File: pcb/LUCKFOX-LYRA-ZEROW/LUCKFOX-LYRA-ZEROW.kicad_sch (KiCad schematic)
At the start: 73 parts, among them J1 Conn_01x07, J2 Conn_01x05, J3 Conn_01x07, J4 Conn_01x05, J5 Conn_01x05, U1 Luckfox_Lyra_Zero_W, U10 RAA211403, U11 SN74LVC1G74DCUT, U12 74LVC2G66, U13 TPS3839G33DBZT, U14 74AUP2G34GW,125, U2 CORE52840, U3 MAX3051, U4 MCP2518FD-xQBB, U5 MAX3051, U6 MAX3051, U7 MCP2518FD-xQBB, U8 MAX3051, U9 74AUP2G34GW,125, Y4 Crystal_GND24_Small, Y5 Crystal_GND24_Small

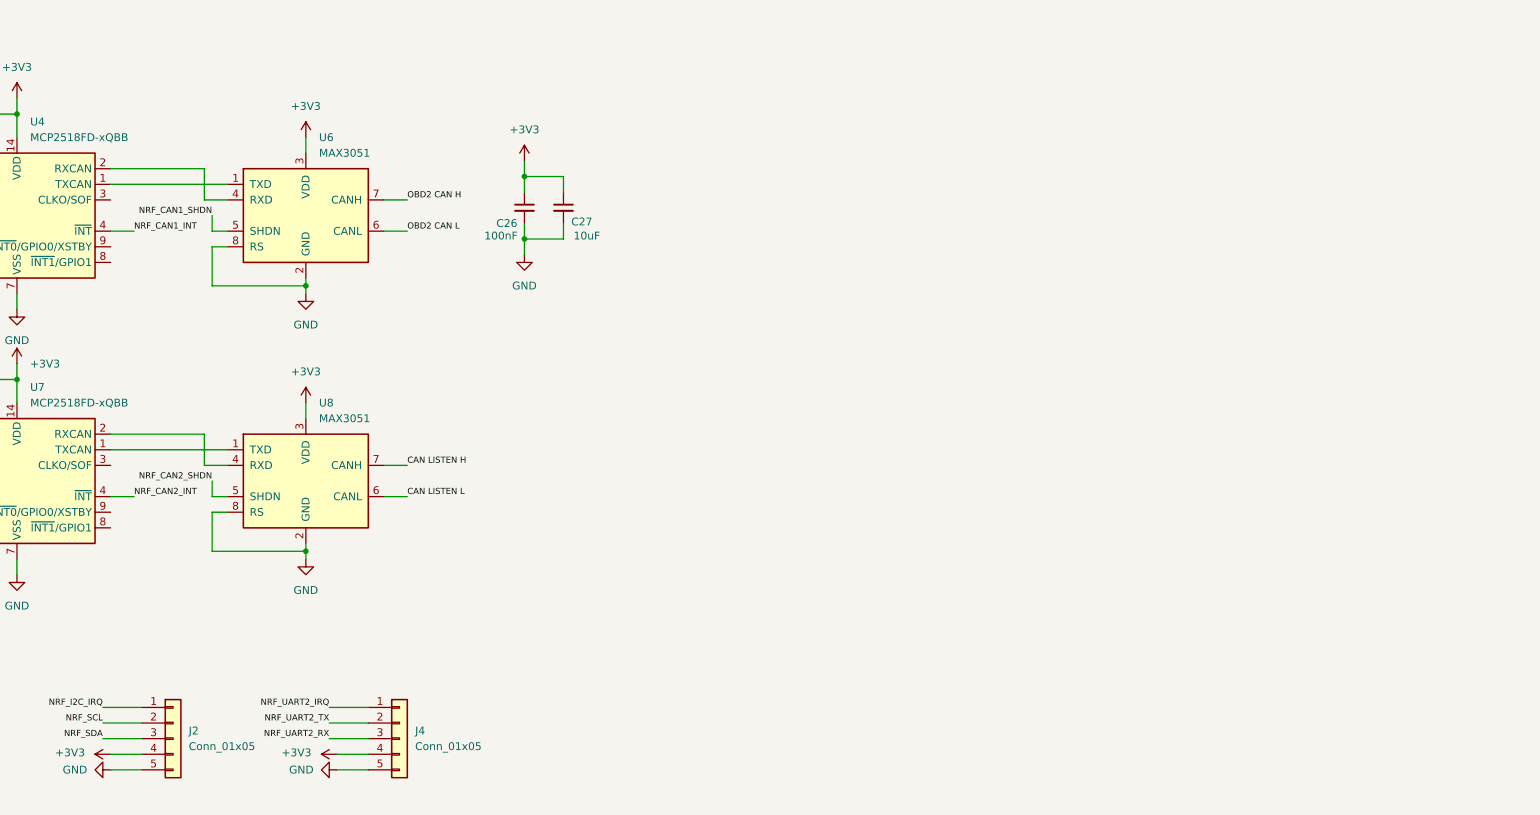
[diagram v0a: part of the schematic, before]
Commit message: fix mcp on pcb
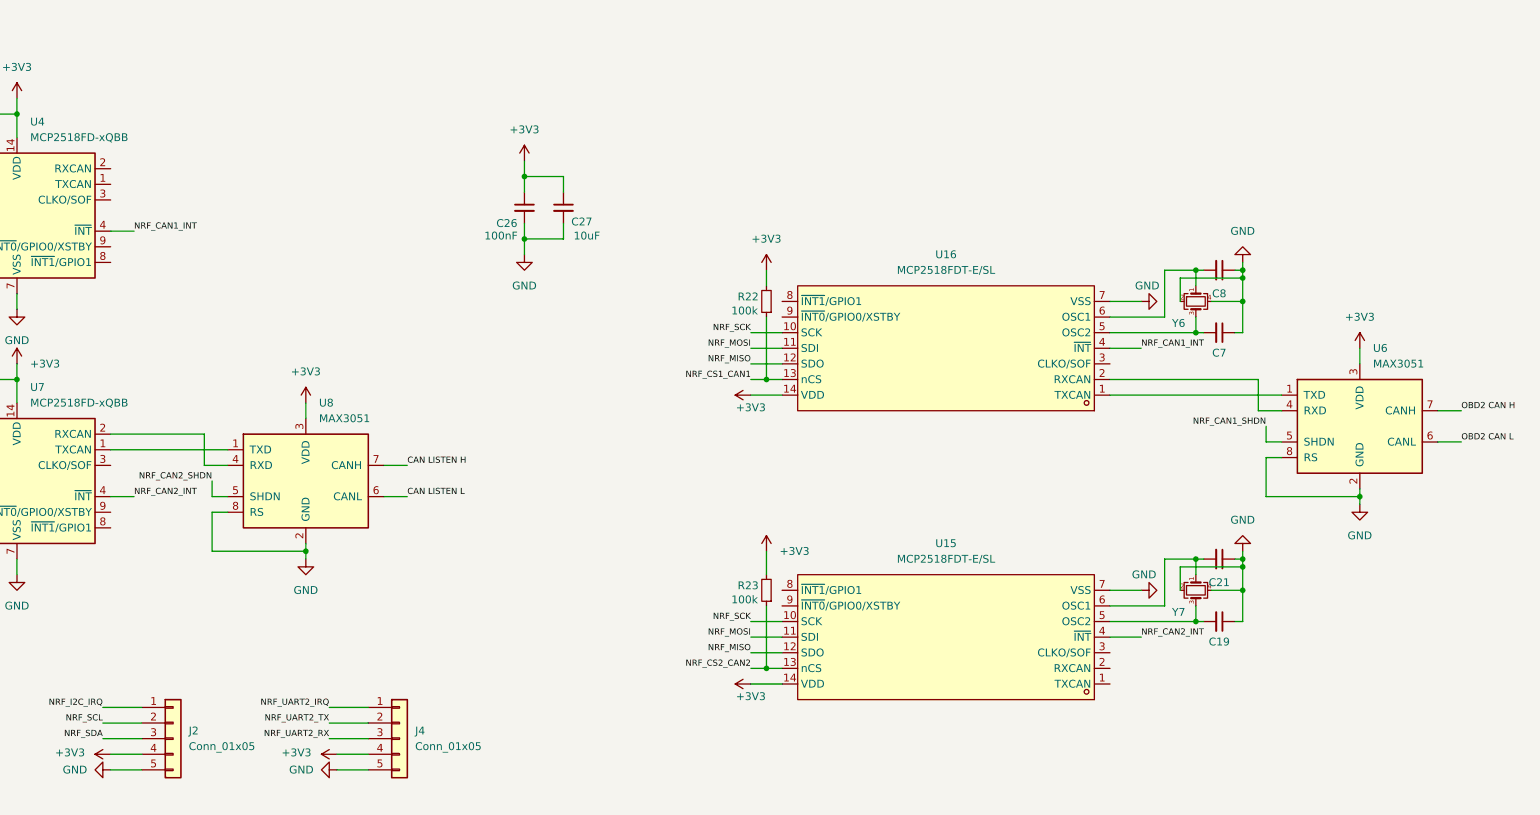
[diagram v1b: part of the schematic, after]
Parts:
- added C19, C21, C7, C8: 22pF, Capacitor_SMD:C_0805_2012Metric, symbol Device:C_Small
- added R22, R23: (150k/1%_0805), Resistor_SMD:R_0805_2012Metric_Pad1.20x1.40mm_HandSolder, symbol ETH3:R_small_PG
- added U15, U16: MCP2518FDT-E/SL, MCP2518FD:SOIC-14_L8.7-W3.9-P1.27-LS6.0-BL, symbol MCP2518FD:MCP2518FDT-E_SL
- added Y6, Y7: Crystal_GND24_Small, Crystal:Crystal_SMD_3225-4Pin_3.2x2.5mm, symbol Device:Crystal_GND24_Small
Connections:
- net +3V3: now also R22.2, R23.2, U15.14 (VDD), U16.14 (VDD)
- net GND: now also C19.1, C21.1, C7.1, C8.1, U15.7 (VSS), U16.7 (VSS), Y6.2, Y6.4, Y7.2, Y7.4
- net NRF_CAN1_INT: now also U16.4 (~{INT})
- net NRF_CAN2_INT: now also U15.4 (~{INT})
- net NRF_CS1_CAN1: now also R22.1, U16.13 (nCS)
- net NRF_CS2_CAN2: now also R23.1, U15.13 (nCS)
- net NRF_MISO: now also U15.12 (SDO), U16.12 (SDO)
- net NRF_MOSI: now also U15.11 (SDI), U16.11 (SDI)
- net NRF_SCK: now also U15.10 (SCK), U16.10 (SCK)
- net at U6.1 (TXD): now also U16.1 (TXCAN); no longer U4.1 (TXCAN)
- net at U6.4 (RXD): now also U16.2 (RXCAN); no longer U4.2 (RXCAN)
- new net: C7.2, U16.5 (OSC2), Y6.3
- new net: C21.2, U15.6 (OSC1), Y7.1
- new net: C19.2, U15.5 (OSC2), Y7.3
- new net: C8.2, U16.6 (OSC1), Y6.1
